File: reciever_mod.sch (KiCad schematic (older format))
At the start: 0 parts

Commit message: adding custom components
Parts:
- added C2: 100pF, symbol C
- added U?: MAX7036, symbol MAX7036
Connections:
- new net: C2.1, U?.8 (MIXIN1)
- new net +3V3: C2.2, U?.12 (DVDD), U?.19 (VDD), U?.4 (AVDD)
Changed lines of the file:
@@
 LIBS:contrib
 LIBS:valves
-LIBS:testpart
+LIBS:CustomComponents
 LIBS:roller_blade-cache
 EELAYER 25 0
@@
 Comment4 ""
 $EndDescr
+$Comp
+L MAX7036 U?
+U 1 1 5A9984C0
+P 2600 2300
+F 0 "U?" H 2600 2300 60  0000 C CNN
+F 1 "MAX7036" H 2600 2300 60  0000 C CNN
+F 2 "" H 2600 2300 60  0001 C CNN
+F 3 "" H 2600 2300 60  0001 C CNN
+	1    2600 2300
+	1    0    0    -1
+$EndComp
+$Comp
+L +3.3V #PWR?
+U 1 1 5A9986F2
+P 1350 2500
+F 0 "#PWR?" H 1350 2350 50  0001 C CNN
+F 1 "+3.3V" H 1350 2640 50  0000 C CNN
+F 2 "" H 1350 2500 50  0001 C CNN
+F 3 "" H 1350 2500 50  0001 C CNN
+	1    1350 2500
+	1    0    0    -1
+$EndComp
+Wire Wire Line
+	1350 2500 1600 2500
+$Comp
+L +3.3V #PWR?
+U 1 1 5A99871A
+P 2800 3600
+F 0 "#PWR?" H 2800 3450 50  0001 C CNN
+F 1 "+3.3V" H 2800 3740 50  0000 C CNN
+F 2 "" H 2800 3600 50  0001 C CNN
+F 3 "" H 2800 3600 50  0001 C CNN
+	1    2800 3600
+	1    0    0    -1
+$EndComp
+Wire Wire Line
+	2800 3600 2800 3300
+$Comp
+L +3.3V #PWR?
+U 1 1 5A99873C
+P 2800 1300
+F 0 "#PWR?" H 2800 1150 50  0001 C CNN
+F 1 "+3.3V" H 2800 1440 50  0000 C CNN
+F 2 "" H 2800 1300 50  0001 C CNN
+F 3 "" H 2800 1300 50  0001 C CNN
+	1    2800 1300
+	1    0    0    -1
+$EndComp
+$Comp
+L C C2
+U 1 1 5A998834
+P 3750 2300
+F 0 "C2" H 3775 2400 50  0000 L CNN
+F 1 "100pF" H 3775 2200 50  0000 L CNN
+F 2 "" H 3788 2150 50  0001 C CNN
+F 3 "" H 3750 2300 50  0001 C CNN
+	1    3750 2300
+	0    -1   -1   0
+$EndComp
+$Comp
+L +3.3V #PWR?
+U 1 1 5A998875
+P 4100 2300
+F 0 "#PWR?" H 4100 2150 50  0001 C CNN
+F 1 "+3.3V" H 4100 2440 50  0000 C CNN
+F 2 "" H 4100 2300 50  0001 C CNN
+F 3 "" H 4100 2300 50  0001 C CNN
+	1    4100 2300
+	1    0    0    -1
+$EndComp
+Wire Wire Line
+	3900 2300 4100 2300
 $EndSCHEMATC

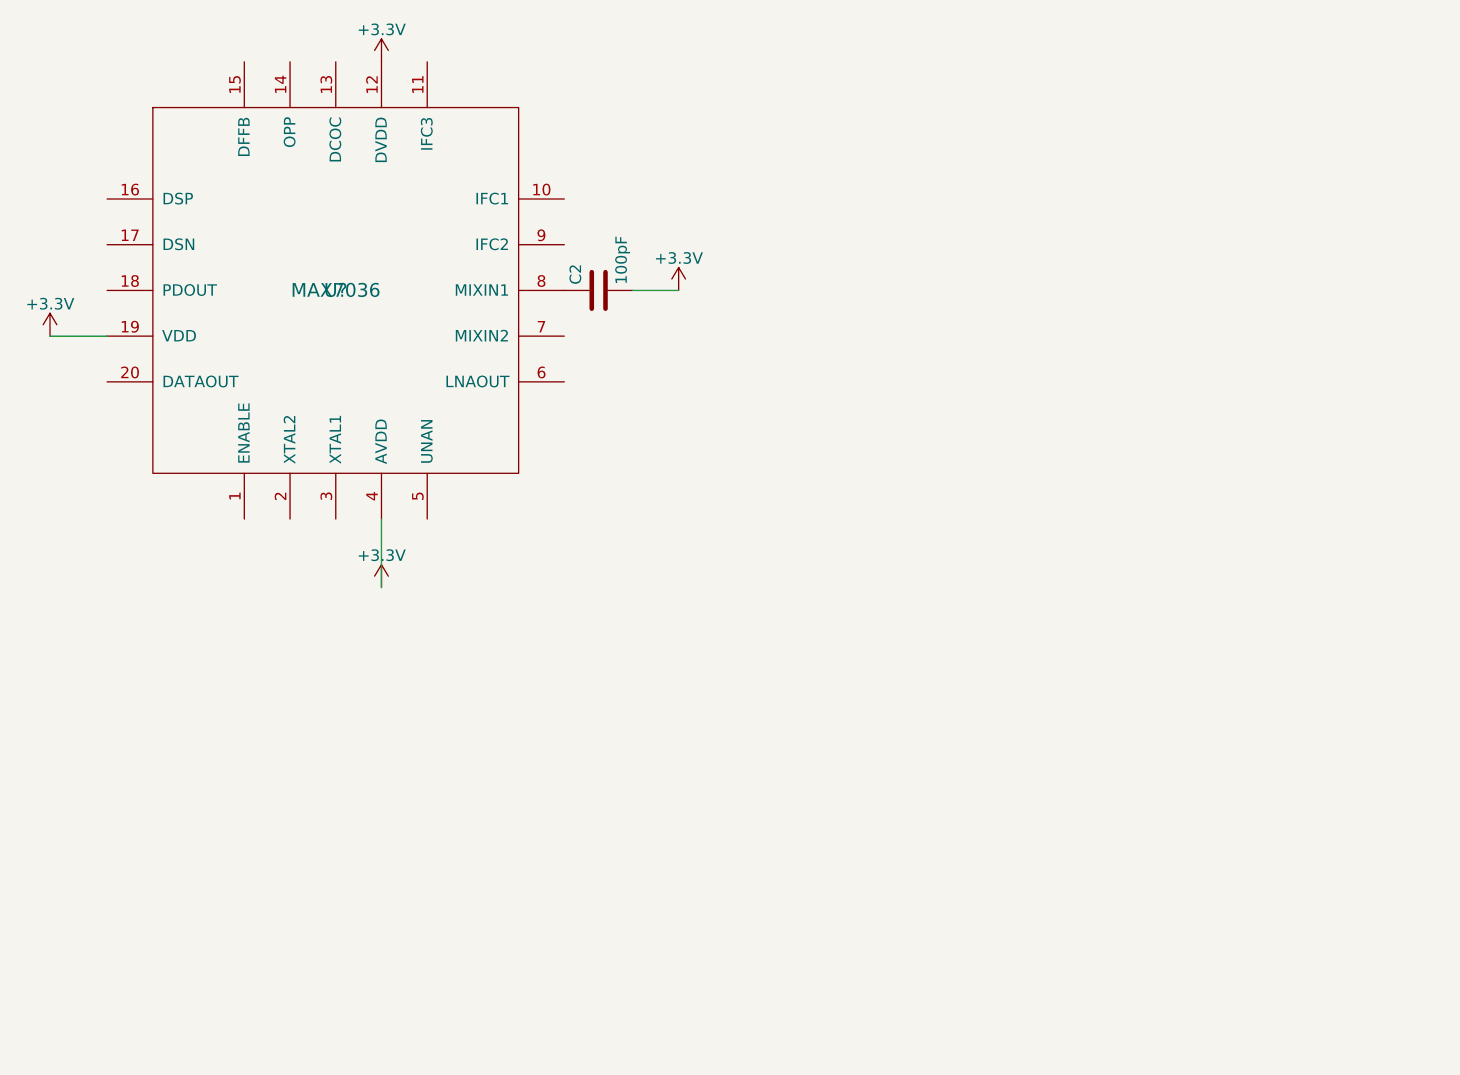
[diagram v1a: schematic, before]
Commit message: commiting reciever
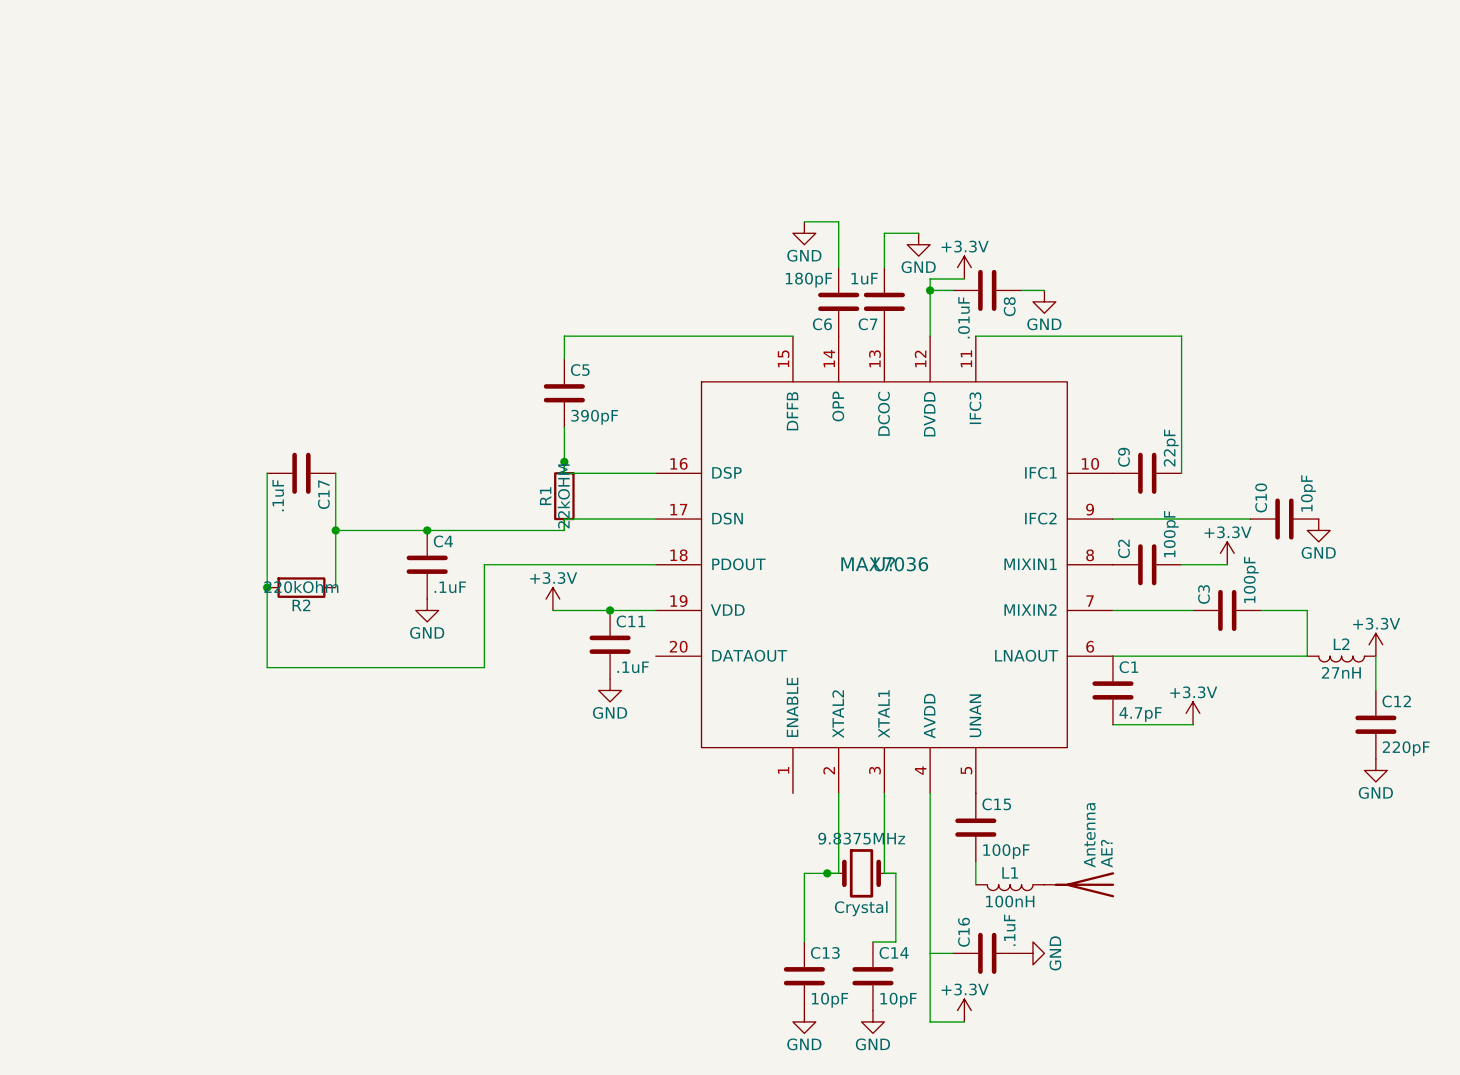
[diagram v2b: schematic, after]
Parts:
- added 9.8375MHz: Crystal, symbol Crystal
- added AE?: Antenna, symbol Antenna
- added C1: 4.7pF, symbol C
- added C10, C13, C14: 10pF, symbol C
- added C11, C16, C17, C4: .1uF, symbol C
- added C12: 220pF, symbol C
- added C15, C3: 100pF, symbol C
- added C5: 390pF, symbol C
- added C6: 180pF, symbol C
- added C7: 1uF, symbol C
- added C8: .01uF, symbol C
- added C9: 22pF, symbol C
- added L1: 100nH, symbol L
- added L2: 27nH, symbol L
- added R1: 22kOHM, symbol R
- added R2: 220kOhm, symbol R
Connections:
- net +3V3: now also C1.2, C11.1, C12.1, C8.2, L2.1
- net at U?.10 (IFC1): now also C9.1
- net at U?.11 (IFC3): now also C9.2
- net at U?.13 (DCOC): now also C7.1
- net at U?.14 (OPP): now also C6.1
- net at U?.15 (DFFB): now also C5.1
- net at U?.16 (DSP): now also C5.2, R1.2
- net at U?.17 (DSN): now also C17.1, C4.1, R1.1, R2.1
- net at U?.18 (PDOUT): now also C17.2, R2.2
- net at U?.2 (XTAL2): now also 9.8375MHz.1, C13.1
- net at U?.3 (XTAL1): now also 9.8375MHz.2, C14.1
- net at U?.5 (UNAN): now also C15.1
- net at U?.6 (LNAOUT): now also C1.1, C3.2, L2.2
- net at U?.7 (MIXIN2): now also C3.1
- net at U?.9 (IFC2): now also C10.1
- new net: C15.2, L1.2
- new net: AE?.1 (A), L1.1
- new net GND: C10.2, C11.2, C12.2, C13.2, C14.2, C16.2, C4.2, C6.2, C7.2, C8.1
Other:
- moved on the sheet: C2, U?
